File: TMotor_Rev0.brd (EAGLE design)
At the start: 56.5 x 66.3 mm, 37 parts, among them U1 INA125U, U2 INA125U

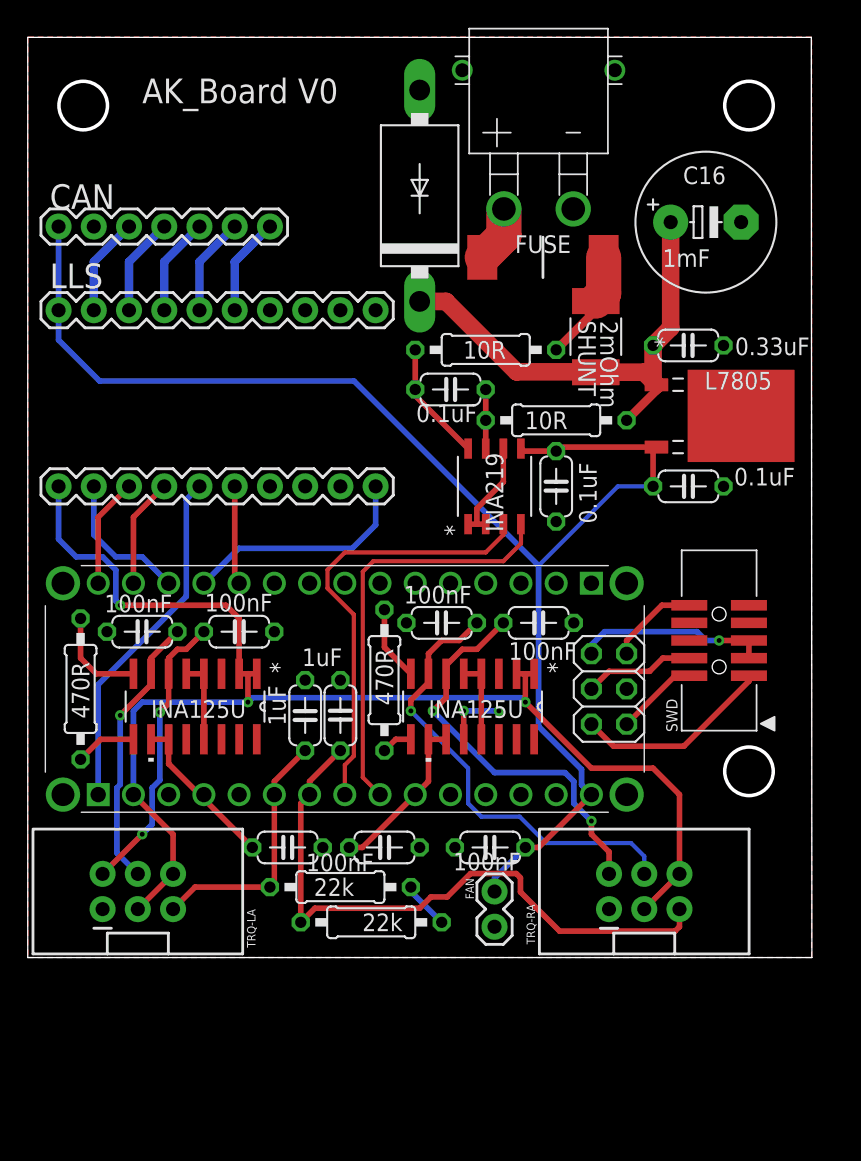
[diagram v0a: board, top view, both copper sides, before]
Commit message: First Rev1 changes
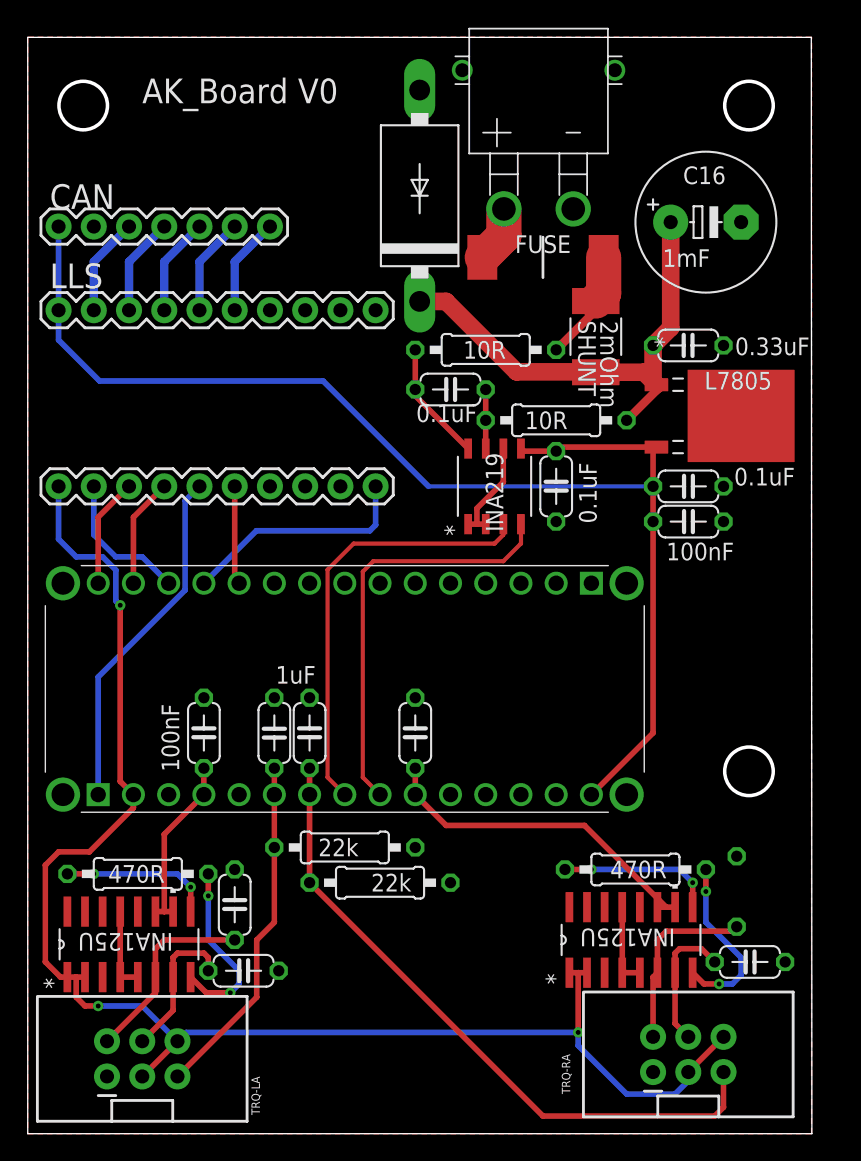
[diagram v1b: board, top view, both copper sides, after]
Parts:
- removed FAN: (no value), SparkFun-Connectors:1X02
- removed POGO: (no value), pinhead:2X03
- removed SWD: 20317, microbuilder:2X05_1.27MM_BOX_POSTS
- moved C7 33.0 mm to (52.1, 8.26), turned to 0 degrees
- moved C15 27.5 mm to (47.6, 40.0), turned to 0 degrees
- moved C13 25.5 mm to (15.6, 7.62), turned to 0 degrees
- moved C8 24.1 mm to (51.1, 13.3), flipped to the bottom, turned to 90 degrees
- moved R14 22.7 mm to (43.8, 14.9), turned to 180 degrees
- moved U2 20.3 mm to (43.5, 9.84), turned to 90 degrees
- moved C14 19.7 mm to (14.9, 12.4), turned to 90 degrees
- moved U1 17.8 mm to (7.30, 9.53), turned to 90 degrees
- moved R16 14.0 mm to (7.94, 14.6), turned to 180 degrees
- moved TRQ-RA 12.2 mm to (47.6, 1.59)
- moved TRQ-LA 12.1 mm to (8.26, 1.27)
- moved C12 10.2 mm to (12.7, 24.8), turned to 90 degrees
- moved C6 8.55 mm to (27.9, 24.8), turned to 90 degrees
- moved R7 2.93 mm to (25.4, 14.0)
- moved R8 2.88 mm to (22.9, 16.5)
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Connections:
- removed net NRESET: POGO.5, SWD.10
- removed net SW3.3V: POGO.2, SWD.1
- removed net SWCLK: POGO.4, SWD.4
- removed net SWDIO: POGO.1, SWD.2
- removed net SWGND: POGO.6, SWD.3, SWD.5
- net GND: no longer FAN.2
- net VIN: no longer FAN.1
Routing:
- net N$9: track 33.0 -> 9.81 mm, vias 1 -> 0
- net N$8: track 29.1 -> 13.2 mm, vias 2 -> 0
- net SW3.3V: track 14.3 -> 0.00 mm
- net SWGND: track 13.9 -> 0.00 mm, vias 1 -> 0
- net A6: track 12.0 -> 24.6 mm
- net VIN: track 101.6 -> 92.4 mm
- net N$11: track 19.9 -> 10.7 mm, vias 1 -> 0
- net N$7: track 2.24 -> 11.4 mm, vias 0 -> 2
- net 3.3V: track 99.6 -> 108.2 mm
- net GND: track 15.6 -> 7.51 mm, vias 2 -> 0
- net SWCLK: track 7.98 -> 0.00 mm
- net N$6: track 5.41 -> 12.8 mm, vias 0 -> 2
- net N$10: track 20.9 -> 14.1 mm, vias 2 -> 0
- net N$12: track 4.41 -> 11.0 mm, vias 0 -> 2
- net A2: track 18.5 -> 25.1 mm
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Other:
- board size 56.5 x 66.3 mm -> 56.5 x 79 mm
